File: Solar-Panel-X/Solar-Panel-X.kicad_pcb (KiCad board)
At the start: 6 copper layers, 48.4 x 48.4 mm, 67 parts, among them J1 FFC2B28-10-G, U1 TSL2561, U2 BQ25570RGRR

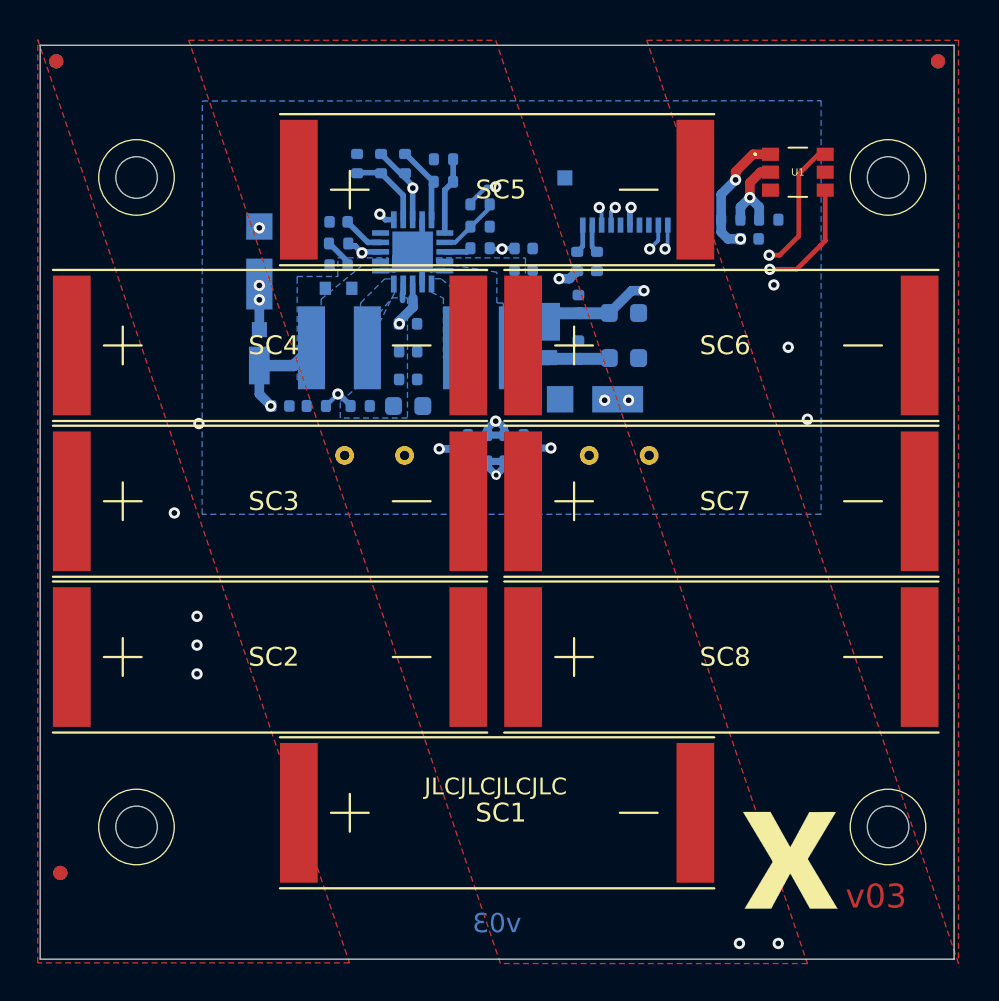
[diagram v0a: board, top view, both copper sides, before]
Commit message: X board updates
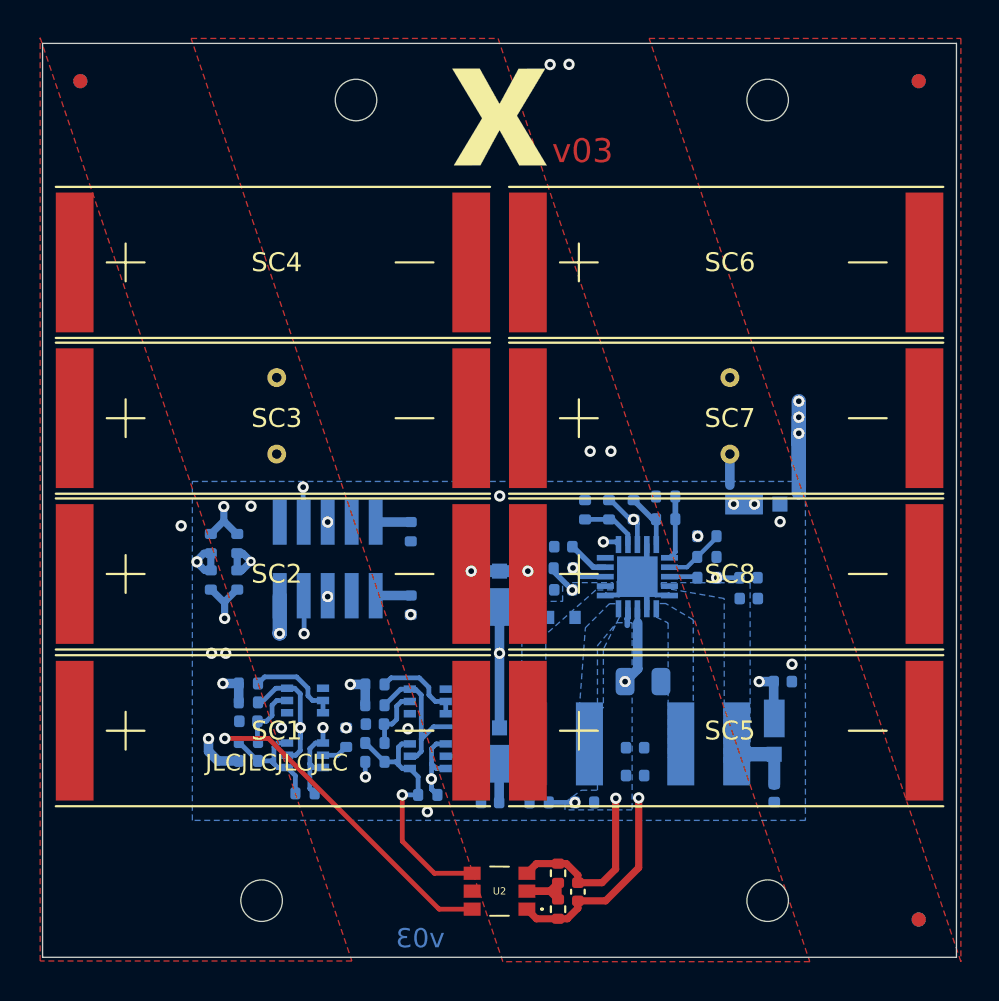
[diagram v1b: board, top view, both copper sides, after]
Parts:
- removed C14: 100uF, Capacitor_SMD:C_0603_1608Metric
- removed the R17 at (110.8, 53.8)
- removed the R18 at (111.9, 53.8)
- added Q1: BSS138DWQ-7, Package_TO_SOT_SMD:SOT-363_SC-70-6, B.Cu at (102.9, 77.2)
- added Q2: MBT2222ADW1T1, Package_TO_SOT_SMD:SOT-363_SC-70-6, B.Cu at (102.9, 80.0)
- added Q3: BSS138DWQ-7, Package_TO_SOT_SMD:SOT-363_SC-70-6, B.Cu at (96.4, 77.1)
- added Q4: MBT2222ADW1T1, Package_TO_SOT_SMD:SOT-363_SC-70-6, B.Cu at (96.4, 80.0)
- added R20: 680, Resistor_SMD:R_0402_1005Metric, B.Cu at (105.0, 79.0)
- added R21: 100K, Resistor_SMD:R_0402_1005Metric, B.Cu at (100.1, 76.2)
- added R22: 0, Resistor_SMD:R_0402_1005Metric, B.Cu at (102.9, 82.1)
- added R23: 0, Resistor_SMD:R_0402_1005Metric, B.Cu at (96.4, 82.0)
- added R24: 10K, Resistor_SMD:R_0402_1005Metric, B.Cu at (100.1, 77.3)
- added R25: 10K, Resistor_SMD:R_0402_1005Metric, B.Cu at (100.1, 80.3)
- added R26: 200K, Resistor_SMD:R_0402_1005Metric, B.Cu at (100.1, 79.3)
- added R27: 680, Resistor_SMD:R_0402_1005Metric, B.Cu at (98.6, 79.0)
- added R28: 100K, Resistor_SMD:R_0402_1005Metric, B.Cu at (93.4, 76.2)
- added R29: 10K, Resistor_SMD:R_0402_1005Metric, B.Cu at (93.4, 77.2)
- added R3: 0, Resistor_SMD:R_0402_1005Metric, B.Cu at (102.0, 72.0)
- added R30: 10K, Resistor_SMD:R_0402_1005Metric, B.Cu at (93.4, 80.3)
- added R31: 200K, Resistor_SMD:R_0402_1005Metric, B.Cu at (93.4, 79.3)
- added R4: 0, Resistor_SMD:R_0402_1005Metric, B.Cu at (102.0, 68.2)
- C1: renamed from C5; value 0.1uF -> 1uF; moved to F.Cu
- C11: value 100uF -> 0.1uF; footprint Capacitor_SMD:C_0603_1608Metric -> Capacitor_SMD:C_0402_1005Metric
- C12: value 100uF -> 10nF; footprint Capacitor_SMD:C_0603_1608Metric -> Capacitor_SMD:C_0402_1005Metric
- C13: value 0.1uF -> 10nF
- C5: renamed from C6; footprint Capacitor_SMD:C_0402_1005Metric -> Capacitor_SMD:C_0805_2012Metric
- C6: renamed from C1; value 1.0uF -> 1uF
- D1: value SDM20U40-7 -> SZMM5Z5V1T1G
- D4, D5: value SBDiode -> MSS1P4-M3_89A; footprint solarpanels:SB Diode -> solarpanels:MICROSMP
- H1, H2, H3, H4: moved to B.Cu
- J1: value FFC2B28-10-G -> TODO; footprint solarpanels:GCT_FFC2B28-10-G -> Connector_PinHeader_1.27mm:PinHeader_2x05_P1.27mm_Vertical_SMD
- R1: renamed from R12; moved to F.Cu
- R2: renamed from R13; moved to F.Cu
- moved REF** 45.5 mm to (128.9, 88.7) (x2)
- moved REF** 42.3 mm to (106.7, 47.7)
- moved U2 41.2 mm to (106.7, 87.2), turned to 180 degrees
- moved H2 40.2 mm to (99.1, 45.3), turned to 180 degrees
- moved H4 38.8 mm to (120.9, 87.7), turned to 180 degrees
- moved R1 37.6 mm to (109.8, 88.2), turned to -90 degrees
- moved R2 36.4 mm to (109.8, 86.2), turned to -90 degrees
- moved C1 35.8 mm to (110.8, 87.2), turned to -90 degrees
- moved H1 33.7 mm to (120.9, 45.3), turned to 180 degrees
- moved H3 33.4 mm to (94.1, 87.7), turned to 180 degrees
- moved SC5 31.1 mm to (108.2, 78.7)
- moved C13 28.2 mm to (93.4, 78.2), turned to 180 degrees
- moved D3 27.5 mm to (120.3, 66.7), turned to 0 degrees
- moved C10 25.7 mm to (121.2, 82.0), turned to -90 degrees
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- renumbered C8 to C7, C7 to C8, R2 to R12, R3 to R13, R4 to R17, R19 to R18, R1 to R19, U2 to U1, U1 to U2
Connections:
- C11 pad 1: Net-(C11-Pad1) -> +3V3
- C12 pad 1: Net-(C10-Pad1) -> Net-(C12-Pad1)
- C13 pad 1: +3V3 -> Net-(C13-Pad1)
- C7 pad 1: Net-(C11-Pad1) -> Net-(C7-Pad1)
- C9 pad 1: Net-(C11-Pad1) -> Net-(C7-Pad1)
- D3 pad 1: VSOLAR -> Net-(D3-Pad1)
- D3 pad 2: /VSOLAR_FULL -> GND
- D4 pad 2: Net-(D4-Pad2) -> Net-(D3-Pad1)
- D5 pad 1: Net-(D4-Pad2) -> VSOLAR
- D5 pad 2: GND -> /VSOLAR_FULL
- J1 pad 10: COIL_P -> GND
- J1 pad 3: SDA1 -> BURN1
- J1 pad 4: SCL1 -> BURN2
- J1 pad 5: BURN1 -> COIL_P
- J1 pad 6: +3V3 -> COIL_N
- J1 pad 7: GND -> SDA2
- J1 pad 8: GND -> SCL2
- J1 pad 9: COIL_N -> +3V3
- R16 pad 1: Net-(C11-Pad1) -> Net-(C7-Pad1)
- SC1 pad 2: Net-(D4-Pad2) -> Net-(D3-Pad1)
- SC2 pad 2: Net-(D4-Pad2) -> Net-(D3-Pad1)
- SC3 pad 2: Net-(D4-Pad2) -> Net-(D3-Pad1)
- SC4 pad 2: Net-(D4-Pad2) -> Net-(D3-Pad1)
- SC5 pad 1: Net-(D4-Pad2) -> Net-(D3-Pad1)
- SC6 pad 1: Net-(D4-Pad2) -> Net-(D3-Pad1)
- SC7 pad 1: Net-(D4-Pad2) -> Net-(D3-Pad1)
- SC8 pad 1: Net-(D4-Pad2) -> Net-(D3-Pad1)
- TP1 pad 1: +3V3 -> VSOLAR
- TP3 pad 1: VBAT -> +3V3
- TP4 pad 1: VSOLAR -> VBAT
- U1 pad 19: Net-(C11-Pad1) -> Net-(C7-Pad1)
- U2 pad 4: SCL1 -> SCL_LS
- U2 pad 6: SDA1 -> SDA_LS
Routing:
- net /coil: track 12851.8 -> 13245.7 mm, vias 6 -> 5
- net SCL2: track 0.00 -> 25.7 mm, vias 0 -> 2
- net SDA_LS: track 0.00 -> 24.0 mm, vias 0 -> 1
- net GND: track 9.09 -> 28.1 mm, vias 3 -> 11
- net SDA1: track 19.1 -> 0.00 mm, vias 2 -> 0
- net SCL1: track 17.3 -> 0.00 mm, vias 2 -> 0
- net COIL_P: track 23.8 -> 7.60 mm
- net SCL_LS: track 0.00 -> 13.8 mm, vias 0 -> 1
- net Net-(D3-Pad1): track 0.00 -> 13.4 mm, vias 0 -> 6
- net SDA2: track 0.00 -> 12.3 mm, vias 0 -> 2
- net VSOLAR: track 12.2 -> 22.8 mm
- net VBAT: track 20.2 -> 30.7 mm
- net COIL_N: track 21.2 -> 10.7 mm
- net Net-(Q3-Pad6): track 0.00 -> 9.57 mm, vias 0 -> 2
- net Net-(Q1-Pad6): track 0.00 -> 8.89 mm
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- added copper zone on In2.Cu, net +3V3
- added copper zone on In3.Cu, net GND
- added copper zone on B.Cu, net Net-(C7-Pad1)
- added copper zone on F.Cu, net Net-(D3-Pad1)
- removed copper zone on B.Cu, net Net-(C11-Pad1)
- removed copper zone on F.Cu, net Net-(D4-Pad2)
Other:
- board text added: "Cable Pinout 1.BATT_P 2.VUSB 3.BURN1 4.BURN2 5.COIL_P 6.COIL_N 7.SDA 8.SCL 9.+3V3 10.GND"
- board text removed: "1"
- board text removed: "Cable Pinout 1.BATT_P 2.BATT_N 3.SDA 4.SCL 5.BURN 6.3V3 7.GND 8.GND 9.COIL_N 10.COIL_P"
